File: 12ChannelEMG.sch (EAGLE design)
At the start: 45 parts

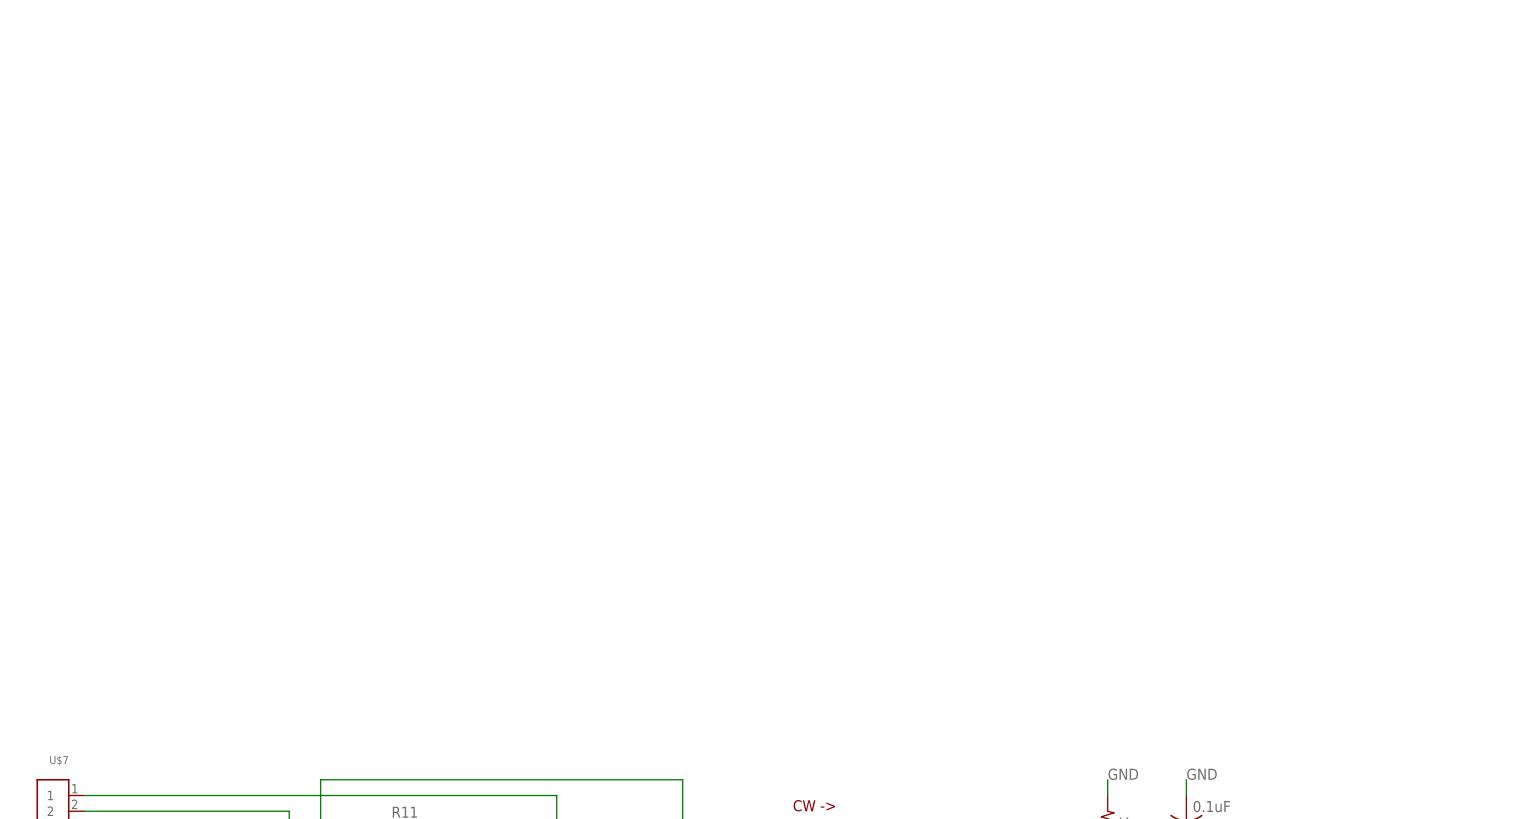
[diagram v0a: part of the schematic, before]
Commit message: Channel 4
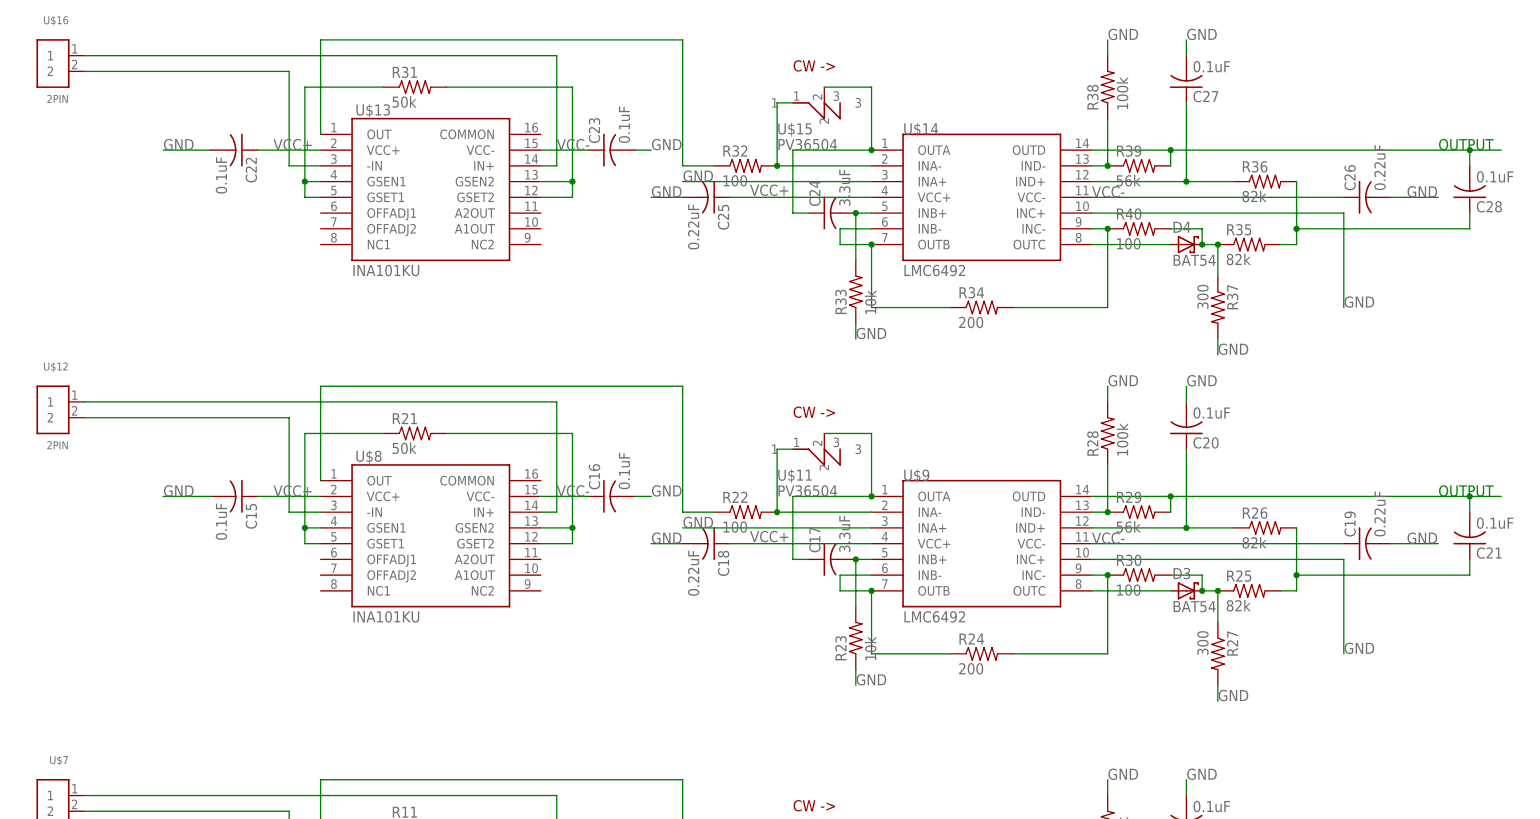
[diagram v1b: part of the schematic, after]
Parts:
- added C15, C16, C20, C21, C22, C23, C27, C28: 0.1uF, resistor:C-USC1206K
- added C17, C24: 3.3uF, resistor:C-USC1206K
- added C18, C19, C25, C26: 0.22uF, rcl:C-USC0603K
- added D3, D4: BAT54, diode:BAT54
- added R21, R31: 50k, rcl:R-US_R0805
- added R22, R30, R32, R40: 100, resistor:R-US_R0603
- added R23, R33: 10k, rcl:R-US_R0603
- added R24, R34: 200, rcl:R-US_R0603
- added R25, R26, R35, R36: 82k, resistor:R-US_R0603
- added R27, R37: 300, resistor:R-US_R0603
- added R28, R38: 100k, resistor:R-US_R0603
- added R29, R39: 56k, resistor:R-US_R0603
- added U$11, U$15: PV36504, 12-ChannelEMG:PV36
- added U$12, U$16: 2PIN, 12-ChannelEMG:2PIN
- added U$13, U$8: INA101KU, 12-ChannelEMG:INA101KUINA101KU
- added U$14, U$9: LMC6492, 12-ChannelEMG:LMC6492
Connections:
- new net N$35: R21.2, U$8.GSEN2, U$8.GSET2
- new net N$36: U$12.2, U$8.-IN
- new net N$37: R22.2, U$11.1, U$9.INA-
- new net N$38: R22.1, U$8.OUT
- new net N$39: C17.1, U$11.2, U$9.OUTA
- new net N$40: C17.2, R23.2, U$9.INB+
- new net N$41: R24.1, U$9.INB-, U$9.OUTB
- new net N$42: R24.2, R30.1, U$9.INC-
- new net N$43: D3.A, U$9.OUTC
- new net N$44: C20.1, R26.1, U$9.IND+
- new net N$45: D3.C, R25.1, R27.1, R30.2
- new net N$46: C21.2, R29.2, U$9.OUTD
- new net N$47: R28.1, R29.1, U$9.IND-
- new net N$48: C21.1, R25.2, R26.2
- new net N$49: R21.1, U$8.GSEN1, U$8.GSET1
- new net N$50: U$12.1, U$8.IN+
- new net N$51: R31.2, U$13.GSEN2, U$13.GSET2
- new net N$52: U$13.-IN, U$16.2
- new net N$53: R32.2, U$14.INA-, U$15.1
- new net N$54: R32.1, U$13.OUT
- new net N$55: C24.1, U$14.OUTA, U$15.2
- new net N$56: C24.2, R33.2, U$14.INB+
- new net N$57: R34.1, U$14.INB-, U$14.OUTB
- new net N$58: R34.2, R40.1, U$14.INC-
- new net N$59: D4.A, U$14.OUTC
- new net N$60: C27.1, R36.1, U$14.IND+
- new net N$61: D4.C, R35.1, R37.1, R40.2
- new net N$62: C28.2, R39.2, U$14.OUTD
- new net N$63: R38.1, R39.1, U$14.IND-
- new net N$64: C28.1, R35.2, R36.2
- new net N$65: R31.1, U$13.GSEN1, U$13.GSET1
- new net N$66: U$13.IN+, U$16.1
- net GND: now also C15.2, C16.2, C18.2, C19.2, C20.2, C22.2, C23.2, C25.2, C26.2, C27.2, R23.1, R27.2, R28.2, R33.1, R37.2, R38.2, U$14.INA+, U$14.INC+, U$9.INA+, U$9.INC+
- net VCC+: now also C15.1, C18.1, C22.1, C25.1, U$13.VCC+, U$14.VCC+, U$8.VCC+, U$9.VCC+
- net VCC-: now also C16.1, C19.1, C23.1, C26.1, U$13.VCC-, U$14.VCC-, U$8.VCC-, U$9.VCC-

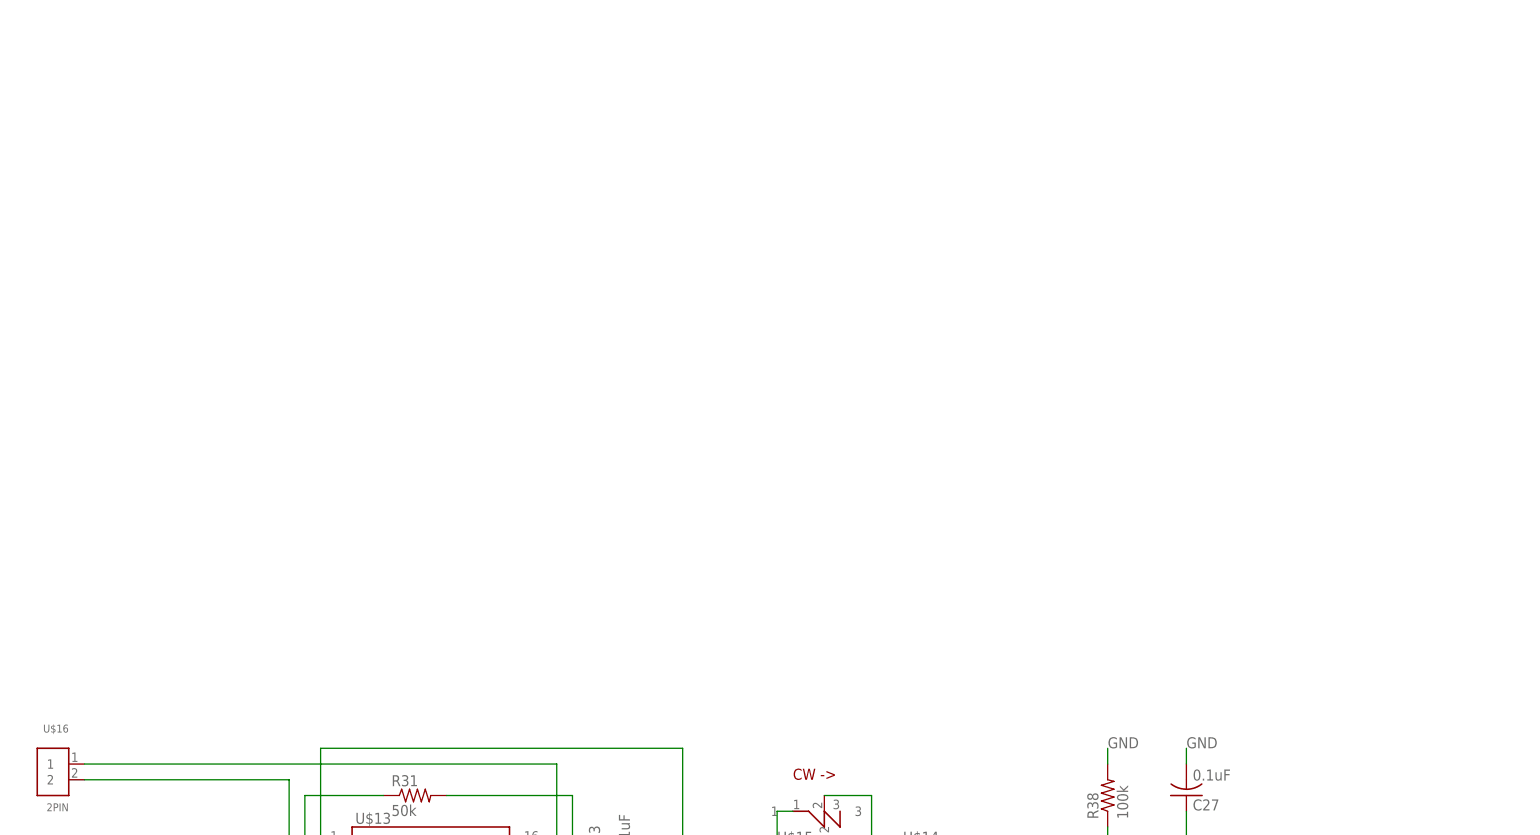
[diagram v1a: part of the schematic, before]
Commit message: Channel 6
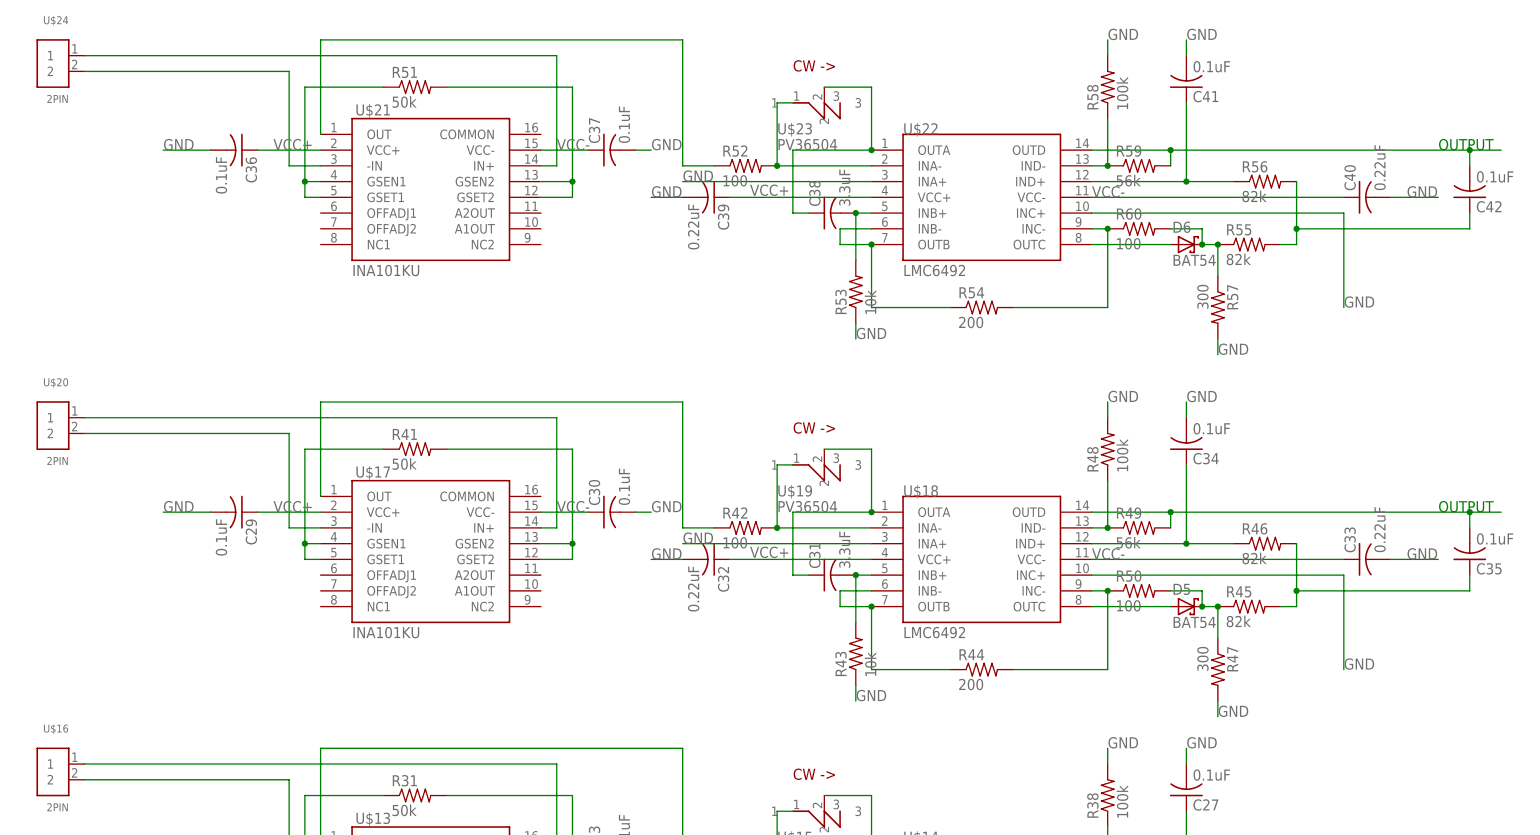
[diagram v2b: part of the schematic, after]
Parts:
- added C29, C30, C34, C35, C36, C37, C41, C42: 0.1uF, resistor:C-USC1206K
- added C31, C38: 3.3uF, resistor:C-USC1206K
- added C32, C33, C39, C40: 0.22uF, rcl:C-USC0603K
- added D5, D6: BAT54, diode:BAT54
- added R41, R51: 50k, rcl:R-US_R0805
- added R42, R50, R52, R60: 100, resistor:R-US_R0603
- added R43, R53: 10k, rcl:R-US_R0603
- added R44, R54: 200, rcl:R-US_R0603
- added R45, R46, R55, R56: 82k, resistor:R-US_R0603
- added R47, R57: 300, resistor:R-US_R0603
- added R48, R58: 100k, resistor:R-US_R0603
- added R49, R59: 56k, resistor:R-US_R0603
- added U$17, U$21: INA101KU, 12-ChannelEMG:INA101KUINA101KU
- added U$18, U$22: LMC6492, 12-ChannelEMG:LMC6492
- added U$19, U$23: PV36504, 12-ChannelEMG:PV36
- added U$20, U$24: 2PIN, 12-ChannelEMG:2PIN
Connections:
- new net N$67: R41.2, U$17.GSEN2, U$17.GSET2
- new net N$68: U$17.-IN, U$20.2
- new net N$69: R42.2, U$18.INA-, U$19.1
- new net N$70: R42.1, U$17.OUT
- new net N$71: C31.1, U$18.OUTA, U$19.2
- new net N$72: C31.2, R43.2, U$18.INB+
- new net N$73: R44.1, U$18.INB-, U$18.OUTB
- new net N$74: R44.2, R50.1, U$18.INC-
- new net N$75: D5.A, U$18.OUTC
- new net N$76: C34.1, R46.1, U$18.IND+
- new net N$77: D5.C, R45.1, R47.1, R50.2
- new net N$78: C35.2, R49.2, U$18.OUTD
- new net N$79: R48.1, R49.1, U$18.IND-
- new net N$80: C35.1, R45.2, R46.2
- new net N$81: R41.1, U$17.GSEN1, U$17.GSET1
- new net N$82: U$17.IN+, U$20.1
- new net N$83: R51.2, U$21.GSEN2, U$21.GSET2
- new net N$84: U$21.-IN, U$24.2
- new net N$85: R52.2, U$22.INA-, U$23.1
- new net N$86: R52.1, U$21.OUT
- new net N$87: C38.1, U$22.OUTA, U$23.2
- new net N$88: C38.2, R53.2, U$22.INB+
- new net N$89: R54.1, U$22.INB-, U$22.OUTB
- new net N$90: R54.2, R60.1, U$22.INC-
- new net N$91: D6.A, U$22.OUTC
- new net N$92: C41.1, R56.1, U$22.IND+
- new net N$93: D6.C, R55.1, R57.1, R60.2
- new net N$94: C42.2, R59.2, U$22.OUTD
- new net N$95: R58.1, R59.1, U$22.IND-
- new net N$96: C42.1, R55.2, R56.2
- new net N$97: R51.1, U$21.GSEN1, U$21.GSET1
- new net N$98: U$21.IN+, U$24.1
- net GND: now also C29.2, C30.2, C32.2, C33.2, C34.2, C36.2, C37.2, C39.2, C40.2, C41.2, R43.1, R47.2, R48.2, R53.1, R57.2, R58.2, U$18.INA+, U$18.INC+, U$22.INA+, U$22.INC+
- net VCC+: now also C29.1, C32.1, C36.1, C39.1, U$17.VCC+, U$18.VCC+, U$21.VCC+, U$22.VCC+
- net VCC-: now also C30.1, C33.1, C37.1, C40.1, U$17.VCC-, U$18.VCC-, U$21.VCC-, U$22.VCC-
